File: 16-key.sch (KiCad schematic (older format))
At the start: 34 parts, among them U1 ProMicro

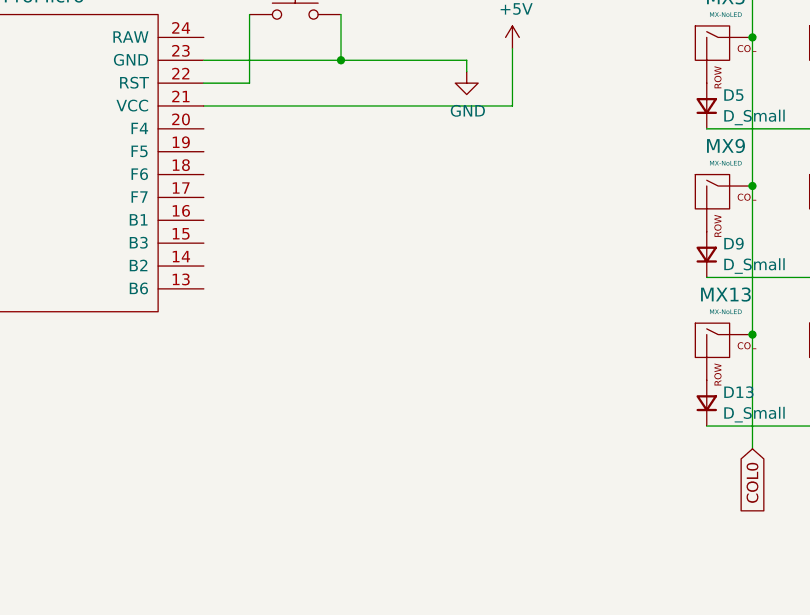
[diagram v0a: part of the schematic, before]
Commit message: basically done
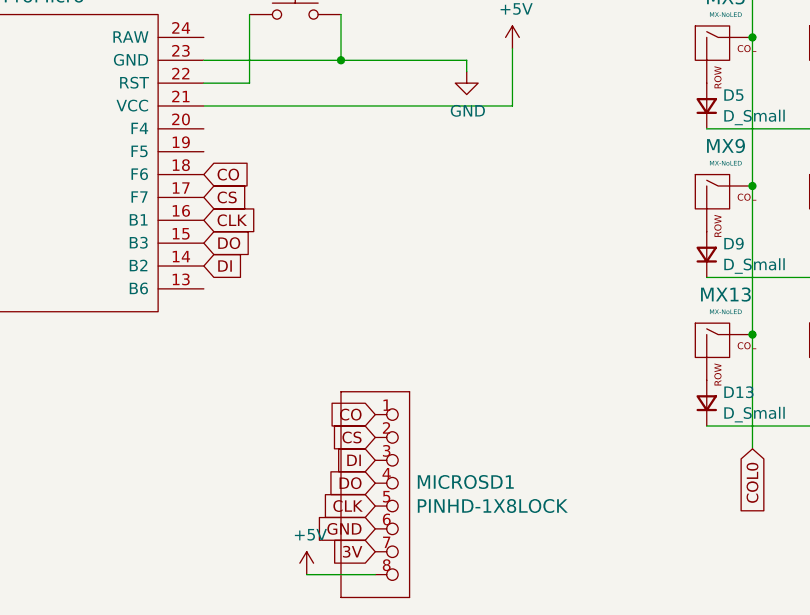
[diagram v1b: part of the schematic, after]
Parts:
- added MICROSD1: PINHD-1X8LOCK, Connector_PinHeader_1.00mm:PinHeader_1x08_P1.00mm_Vertical, symbol 16-key-eagle-import:PINHD-1X8LOCK
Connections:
- net +5V: now also MICROSD1.8
- net GND: now also MICROSD1.6
- net DI: now reaches U1.14 (B2)
- net DI: now also MICROSD1.3
- net DO: now reaches U1.15 (B3)
- net DO: now also MICROSD1.4
- net CLK: now reaches U1.16 (B1)
- net CLK: now also MICROSD1.5
- net CS: now reaches U1.17 (F7)
- net CS: now also MICROSD1.2
- net CO: now reaches U1.18 (F6)
- net CO: now also MICROSD1.1
- new net 3V: MICROSD1.7
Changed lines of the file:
@@
 Text GLabel 6850 3300 3    50   Input ~ 0
 COL3
+Text GLabel 3700 3250 0    50   Input ~ 0
+CS
+Text GLabel 3700 3150 0    50   Input ~ 0
+CO
+Text GLabel 3700 3350 0    50   Input ~ 0
+DI
+Text GLabel 3700 3450 0    50   Input ~ 0
+DO
+Text GLabel 3700 3550 0    50   Input ~ 0
+CLK
+Text GLabel 3700 3650 0    50   Input ~ 0
+GND
+Text GLabel 3700 3750 0    50   Input ~ 0
+3V
+Text GLabel 2950 2400 2    50   Input ~ 0
+DO
+Text GLabel 2950 2500 2    50   Input ~ 0
+DI
+Text GLabel 2950 2300 2    50   Input ~ 0
+CLK
+Text GLabel 2950 2200 2    50   Input ~ 0
+CS
+Text GLabel 2950 2100 2    50   Input ~ 0
+CO
+$Comp
+L 16-key-eagle-import:PINHD-1X8LOCK MICROSD1
+U 1 1 5FFA0D3D
+P 3800 3450
+F 0 "MICROSD1" H 3878 3453 59  0000 L CNN
+F 1 "PINHD-1X8LOCK" H 3878 3348 59  0000 L CNN
+F 2 "Connector_PinHeader_1.00mm:PinHeader_1x08_P1.00mm_Vertical" H 3800 3450 50  0001 C CNN
+F 3 "" H 3800 3450 50  0001 C CNN
+	1    3800 3450
+	1    0    0    -1
+$EndComp
+$Comp
+L power:+5V #PWR0104
+U 1 1 5FFA6FC3
+P 3400 3850
+F 0 "#PWR0104" H 3400 3700 50  0001 C CNN
+F 1 "+5V" H 3415 4023 50  0000 C CNN
+F 2 "" H 3400 3850 50  0001 C CNN
+F 3 "" H 3400 3850 50  0001 C CNN
+	1    3400 3850
+	1    0    0    -1
+$EndComp
+Wire Wire Line
+	3400 3850 3700 3850
 $EndSCHEMATC
